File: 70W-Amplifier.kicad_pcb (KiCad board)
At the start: 2 copper layers, 133.5 x 68 mm, 44 parts, among them J1 RF_OUT, J2 RF_IN, J3 LPF_IN, J4 LPF_OUT, J5 13.8V Input, J6 PTT, J7 Conn_01x02, J8 Conn_01x02, K1 G5V-2, Q1 2N3906-SMD, Q2 IRF530, Q3 IRF530, T1 BN-43-202 1T:2T, T2 Ferrite 1T:3T, U1 L7805

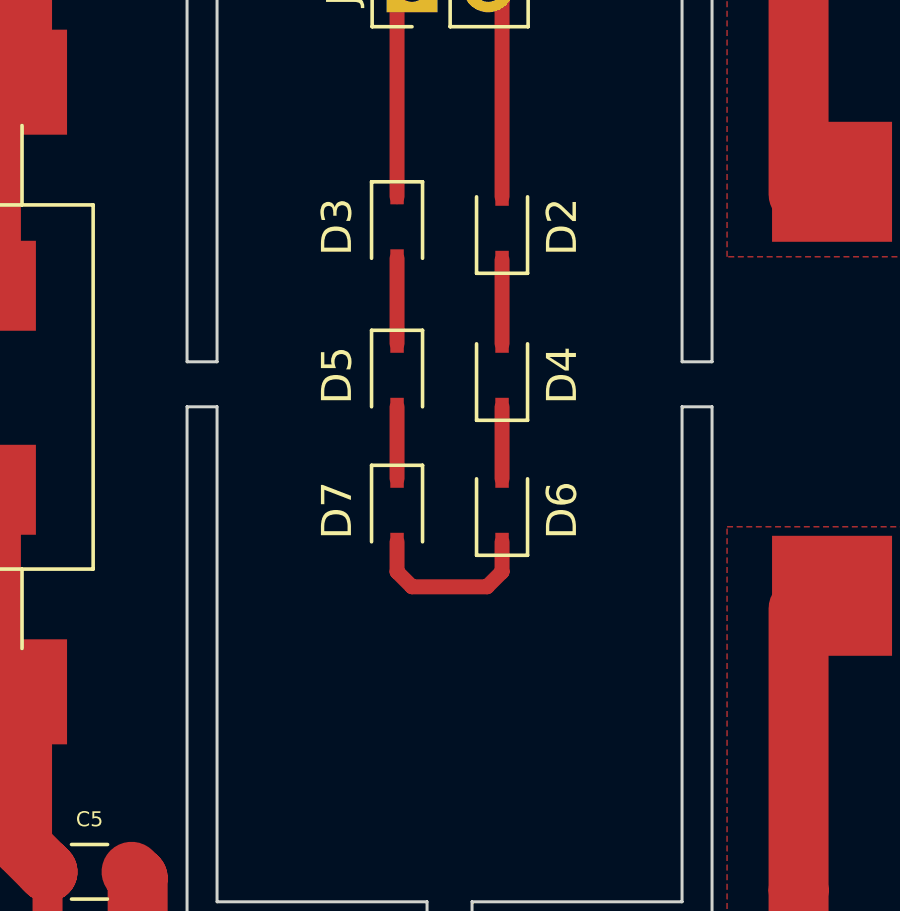
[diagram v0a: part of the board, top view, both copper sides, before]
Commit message: changed diode to sod-123
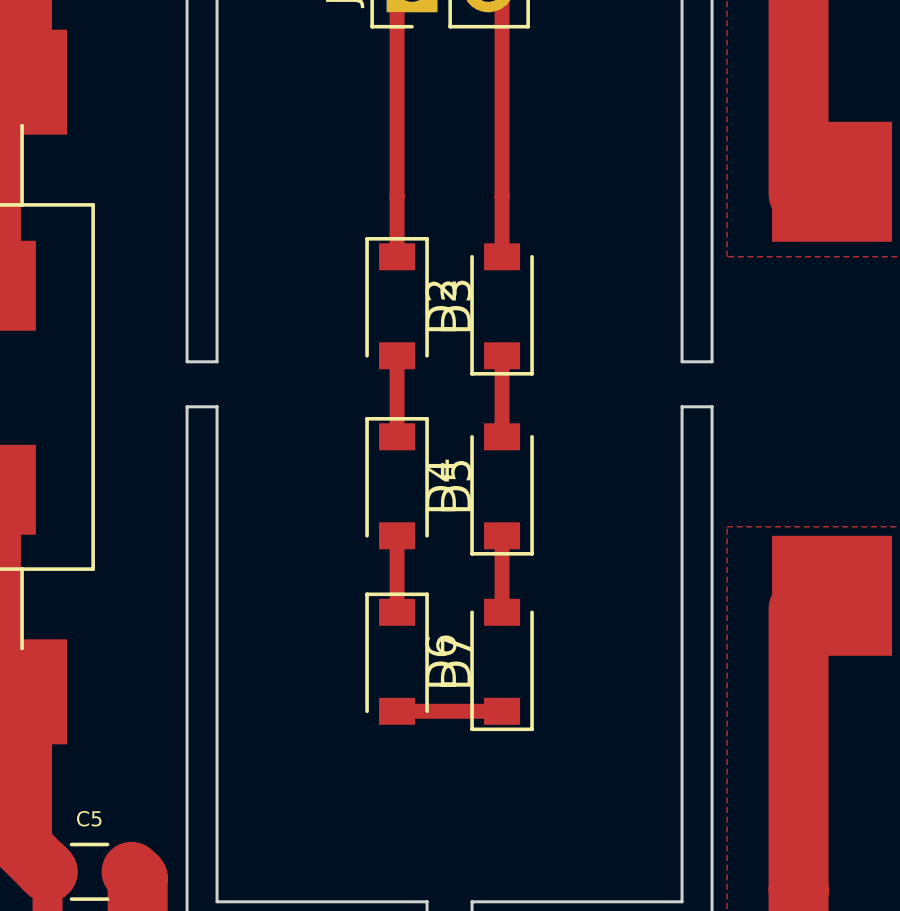
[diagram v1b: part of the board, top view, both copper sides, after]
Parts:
- D2, D3, D4, D5, D6, D7: footprint Diode_SMD:D_SOD-323 -> Diode_SMD:D_SOD-123
- moved D6 5.05 mm to (154.0, 91.0)
- moved D7 5.05 mm to (150.5, 91.0)
- moved D4 3.70 mm to (154.0, 85.2)
- moved D5 3.70 mm to (150.5, 85.2)
- moved D3 2.65 mm to (150.5, 79.2)
- moved D2 2.60 mm to (154.0, 79.2)
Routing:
- net Net-(D6-Pad1): track 5.91 -> 3.50 mm
- net Net-(D3-Pad1): track 7.21 -> 9.21 mm
- net Net-(D2-Pad2): track 7.19 -> 9.19 mm
